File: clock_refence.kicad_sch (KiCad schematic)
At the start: 52 parts, among them J204 REFOUT_AUX_P, J205 REFOUT_AUX_N, J206 RFShield_TwoPieces, J207 REFOUT, J209 DNP, T202 TC2-1T+, U201 Si53301, U202 XC6204B33

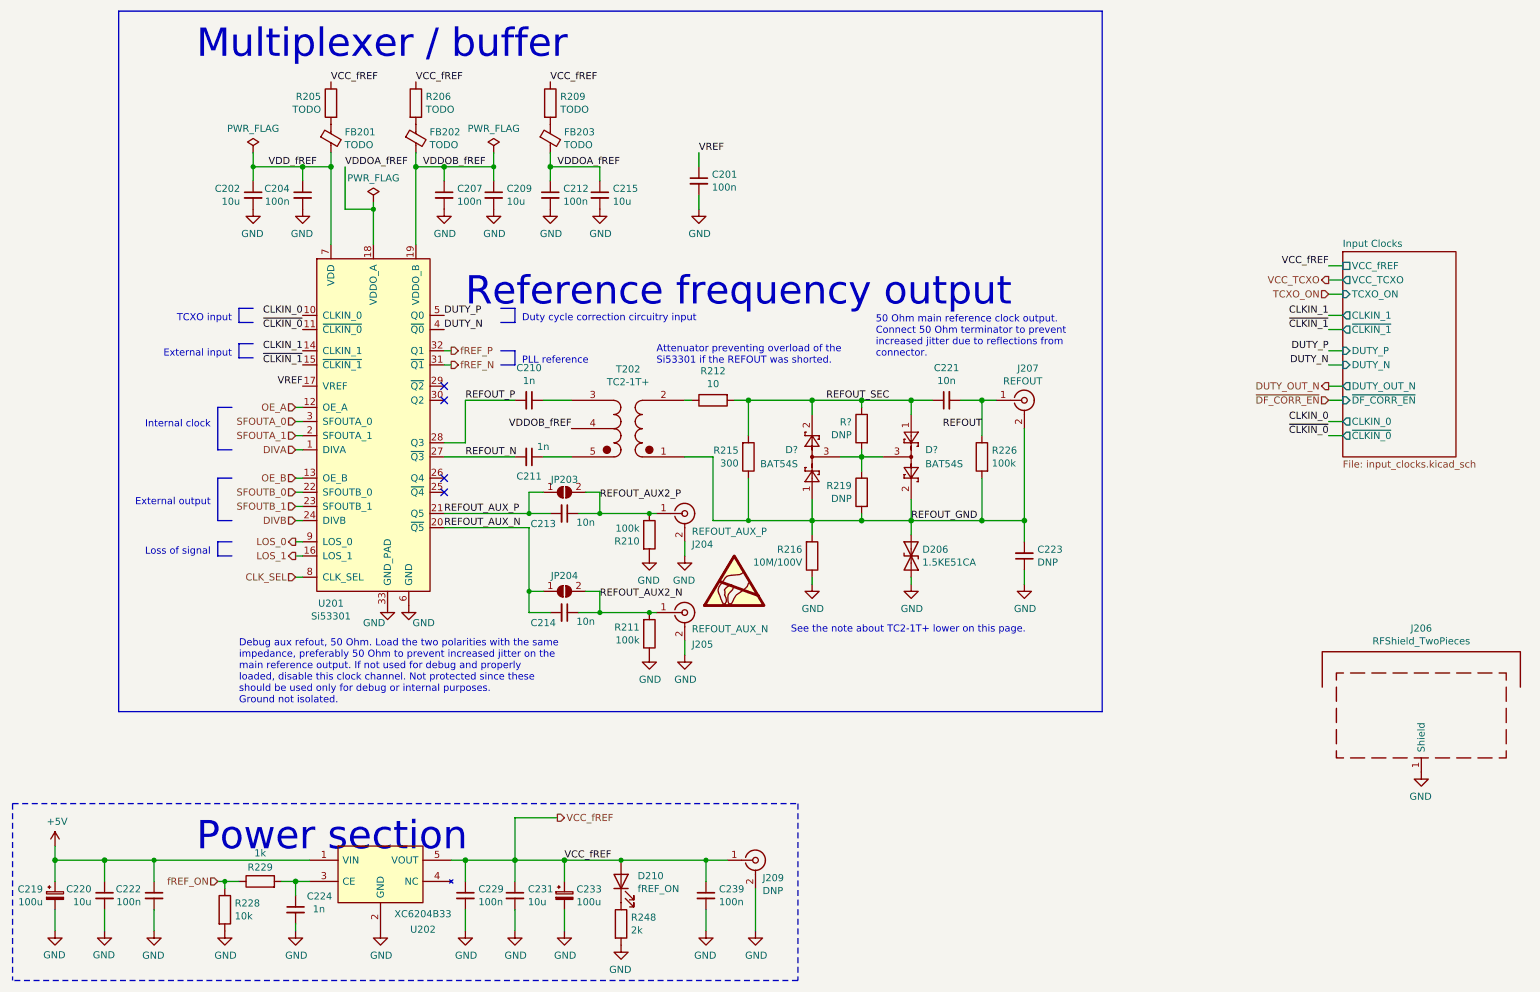
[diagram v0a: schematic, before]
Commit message: Finished schematics
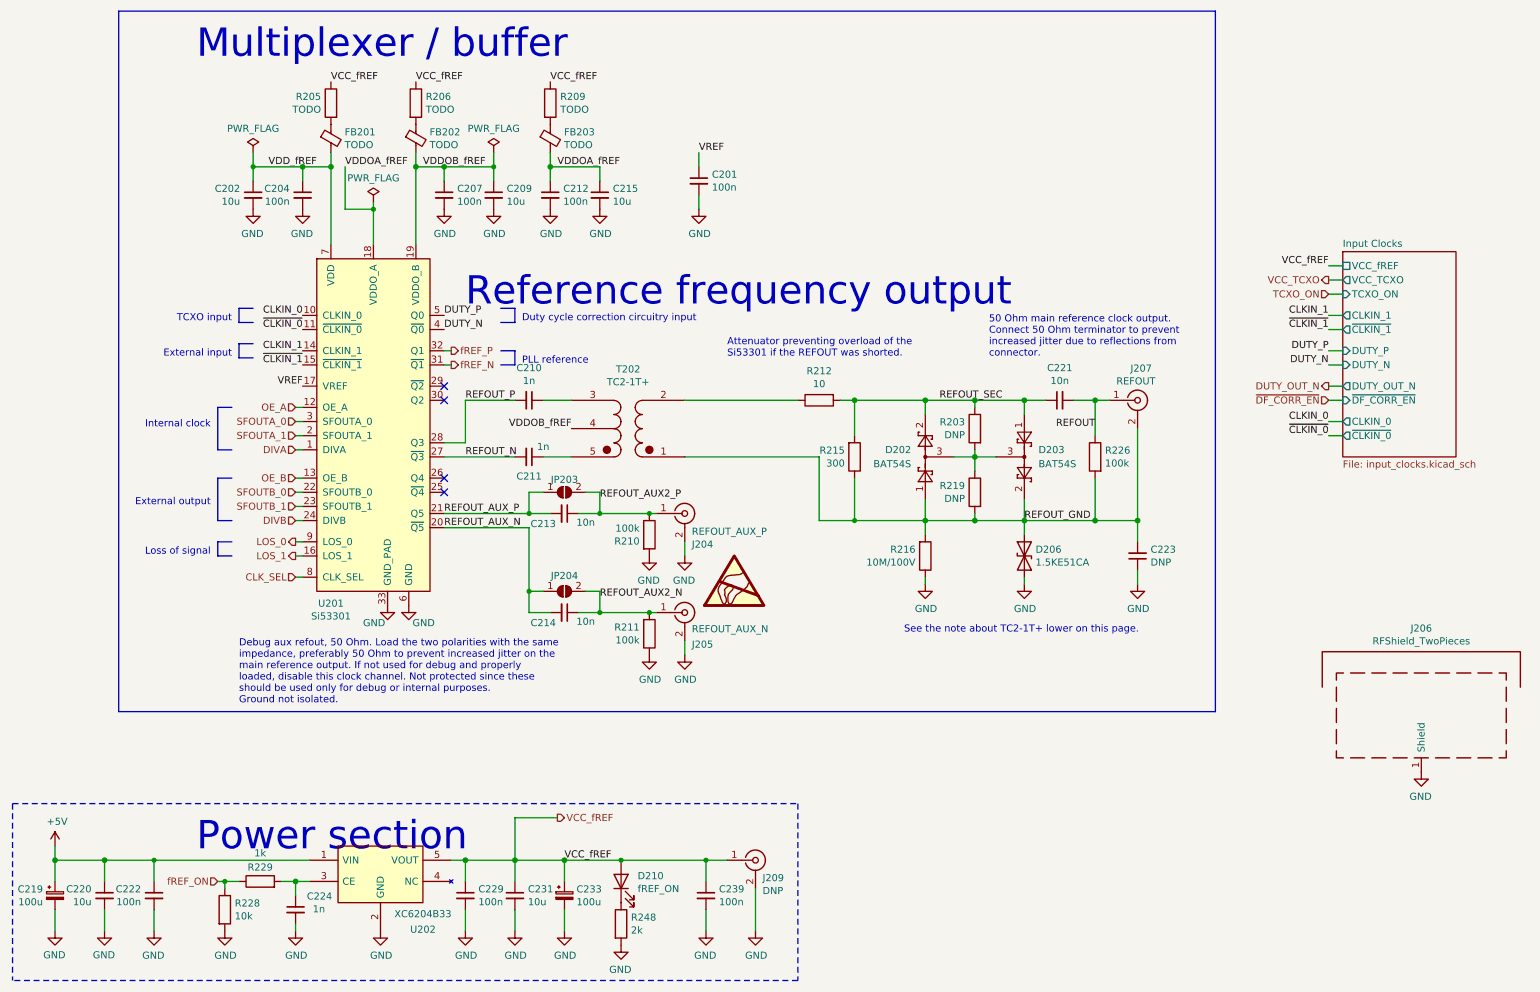
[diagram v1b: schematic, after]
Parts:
- gave numbers to parts that had none: 3
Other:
- moved on the sheet: C221, C223, D202, D203, D206, J207, R203, R212, R215, R216, R219, R226
